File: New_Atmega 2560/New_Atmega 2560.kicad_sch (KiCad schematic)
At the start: 25 parts, among them IC1 1870_LD11117S50CTR, IC2 MC33269D-5.0, J1 Barrel_Jack_Switch, U1 ATmega2560-16A, Y1 Crystal, Y2 16Hz

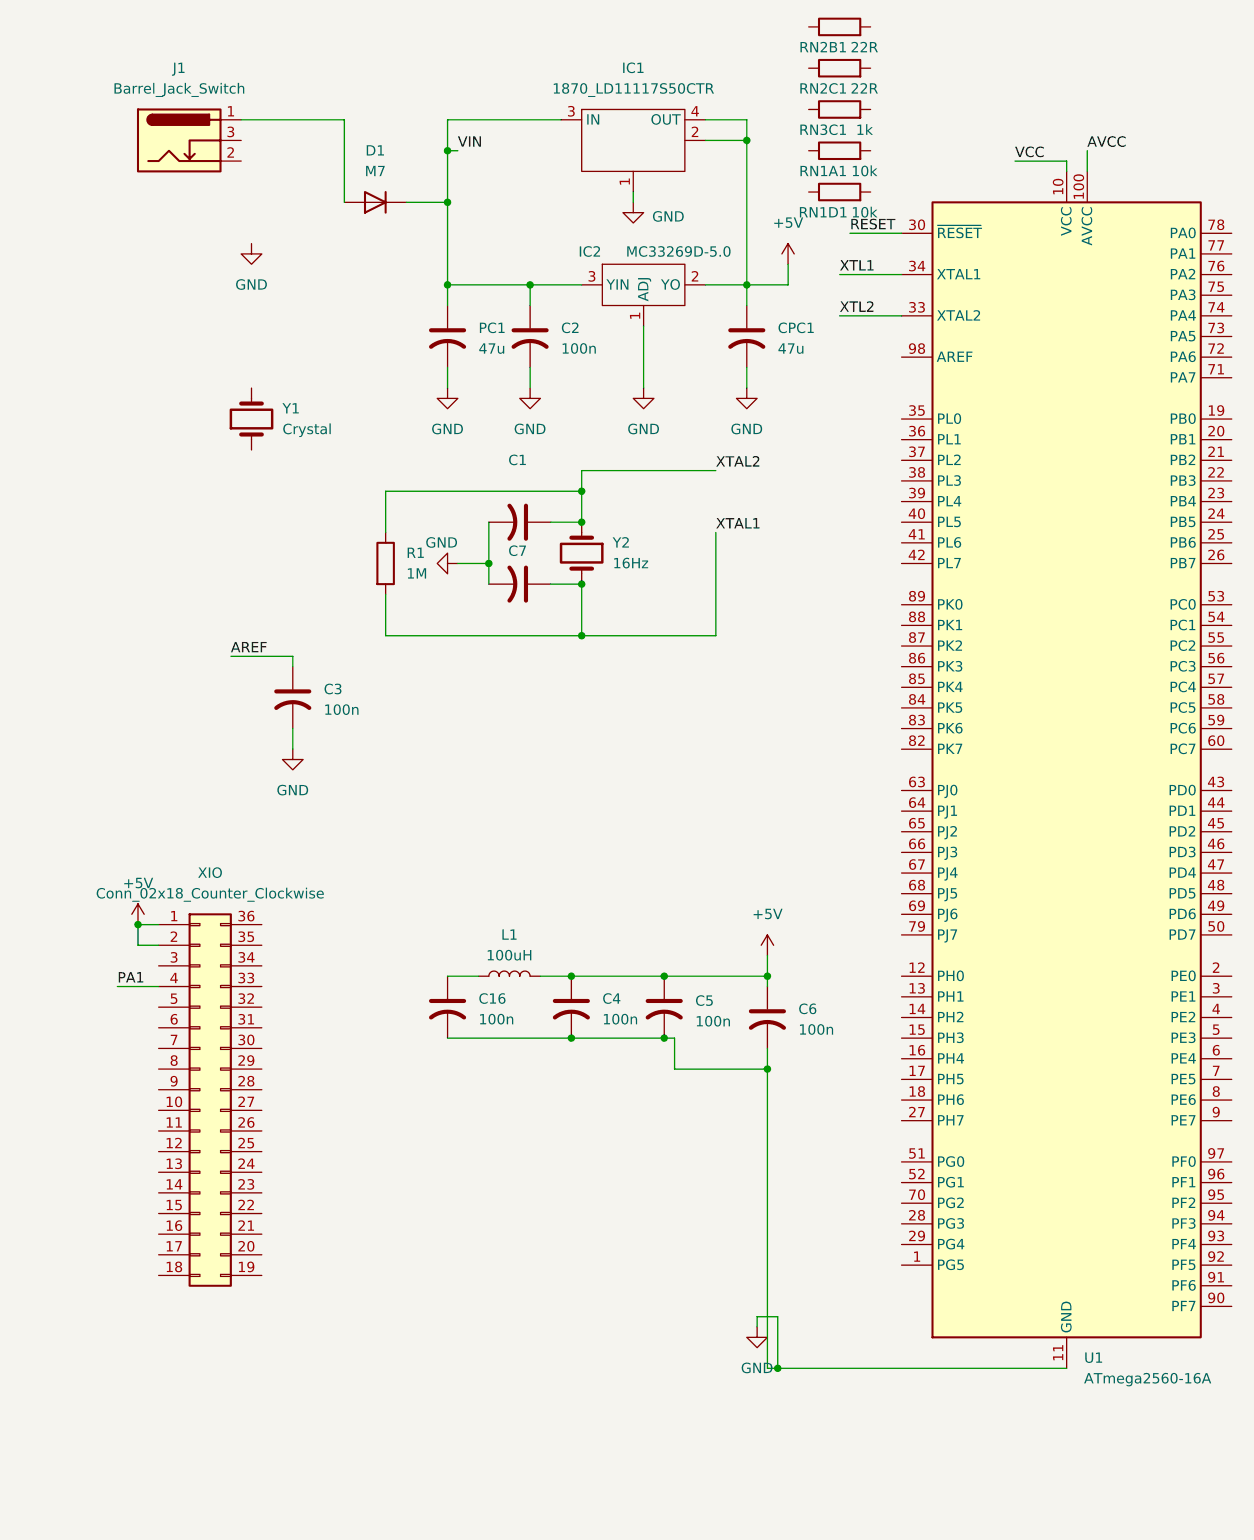
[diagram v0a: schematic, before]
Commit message: Add files via upload
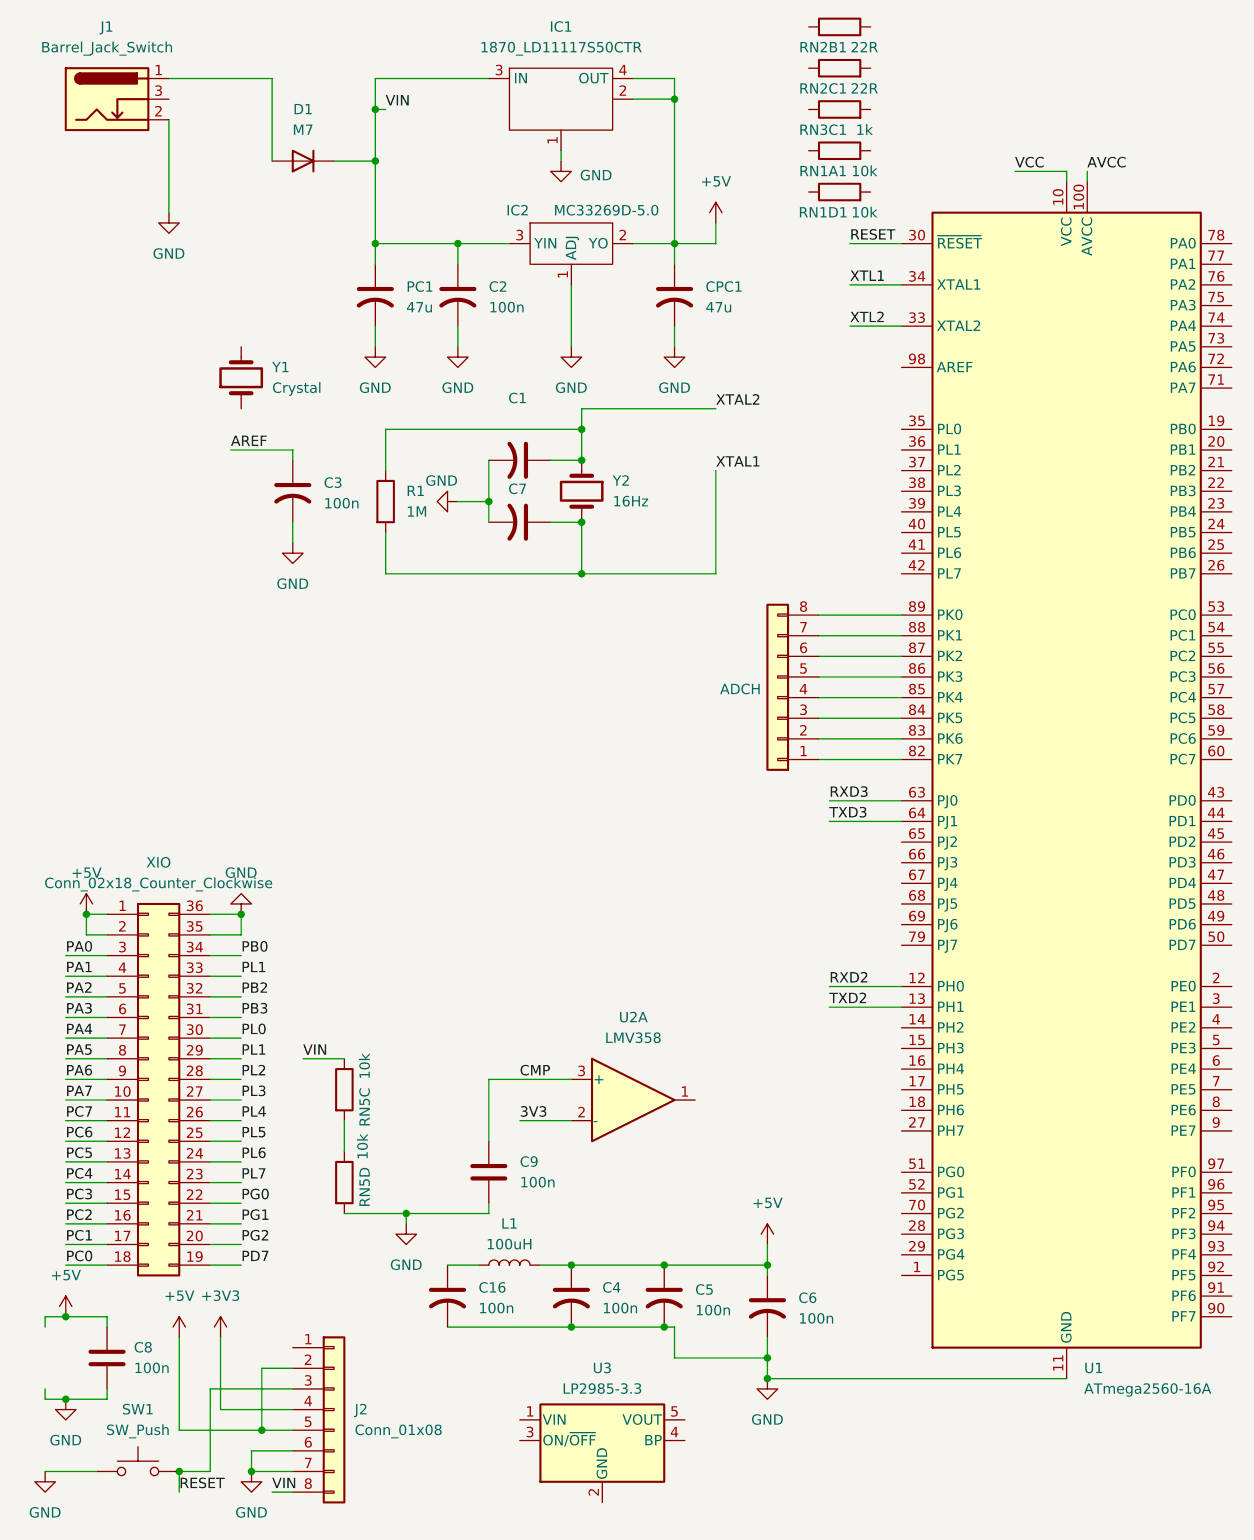
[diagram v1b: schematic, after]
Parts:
- added ADCH: ADCH, symbol Connector_Generic:Conn_01x08
- added C8, C9: 100n, symbol Device:C
- added J2: Conn_01x08, symbol Connector_Generic:Conn_01x08
- added RN5C, RN5D: 10k, symbol Device:R
- added SW1: SW_Push, symbol Switch:SW_Push
- added U2: LMV358, symbol Amplifier_Operational:LMV358
- added U3: LP2985-3.3, Package_TO_SOT_SMD:SOT-23-5, symbol Regulator_Linear:LP2985-3.3
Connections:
- net +5V: now also C8.1, J2.2 (Pin_2), J2.5 (Pin_5)
- net GND: now also J1.2, XIO.35 (Pin_35), XIO.36 (Pin_36), C8.2, C9.2, J2.6 (Pin_6), J2.7 (Pin_7), RN5D.2, SW1.1
- net RESET: now also J2.3 (Pin_3), SW1.2
- net VIN: now also J2.8 (Pin_8), RN5C.1
- net RXD2: now reaches U1.12 (PH0)
- net TXD2: now reaches U1.13 (PH1)
- net RXD3: now reaches U1.63 (PJ0)
- net TXD3: now reaches U1.64 (PJ1)
- net at U1.82 (PK7): now also ADCH.1 (Pin_1)
- net at U1.83 (PK6): now also ADCH.2 (Pin_2)
- net at U1.84 (PK5): now also ADCH.3 (Pin_3)
- net at U1.85 (PK4): now also ADCH.4 (Pin_4)
- net at U1.86 (PK3): now also ADCH.5 (Pin_5)
- net at U1.87 (PK2): now also ADCH.6 (Pin_6)
- net at U1.88 (PK1): now also ADCH.7 (Pin_7)
- net at U1.89 (PK0): now also ADCH.8 (Pin_8)
- net PA7: now reaches XIO.10 (Pin_10)
- net PC7: now reaches XIO.11 (Pin_11)
- net PC6: now reaches XIO.12 (Pin_12)
- net PC5: now reaches XIO.13 (Pin_13)
- net PC4: now reaches XIO.14 (Pin_14)
- net PC3: now reaches XIO.15 (Pin_15)
- net PC2: now reaches XIO.16 (Pin_16)
- net PC1: now reaches XIO.17 (Pin_17)
- net PC0: now reaches XIO.18 (Pin_18)
- net PD7: now reaches XIO.19 (Pin_19)
- net PG2: now reaches XIO.20 (Pin_20)
- net PG1: now reaches XIO.21 (Pin_21)
- net PG0: now reaches XIO.22 (Pin_22)
- net PL7: now reaches XIO.23 (Pin_23)
- net PL6: now reaches XIO.24 (Pin_24)
- net PL5: now reaches XIO.25 (Pin_25)
- net PL4: now reaches XIO.26 (Pin_26)
- net PL3: now reaches XIO.27 (Pin_27)
- net PL2: now reaches XIO.28 (Pin_28)
- net PL1: now reaches XIO.29 (Pin_29)
- net PL1: now also XIO.33 (Pin_33)
- net PA0: now reaches XIO.3 (Pin_3)
- net PL0: now reaches XIO.30 (Pin_30)
- net PB3: now reaches XIO.31 (Pin_31)
- net PB2: now reaches XIO.32 (Pin_32)
- net PB0: now reaches XIO.34 (Pin_34)
- net PA2: now reaches XIO.5 (Pin_5)
- net PA3: now reaches XIO.6 (Pin_6)
- net PA4: now reaches XIO.7 (Pin_7)
- net PA5: now reaches XIO.8 (Pin_8)
- net PA6: now reaches XIO.9 (Pin_9)
- new net: RN5C.2, RN5D.1
- new net +3V3: J2.4 (Pin_4)
- new net 3V3: U2.2 (-)
- new net CMP: C9.1, U2.3 (+)
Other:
- moved on the sheet: C1, C16, C2, C3, C4, C5, C6, C7, CPC1, D1, IC1, IC2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
